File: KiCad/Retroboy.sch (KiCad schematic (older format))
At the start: 1 part, among them J1 1473005-1

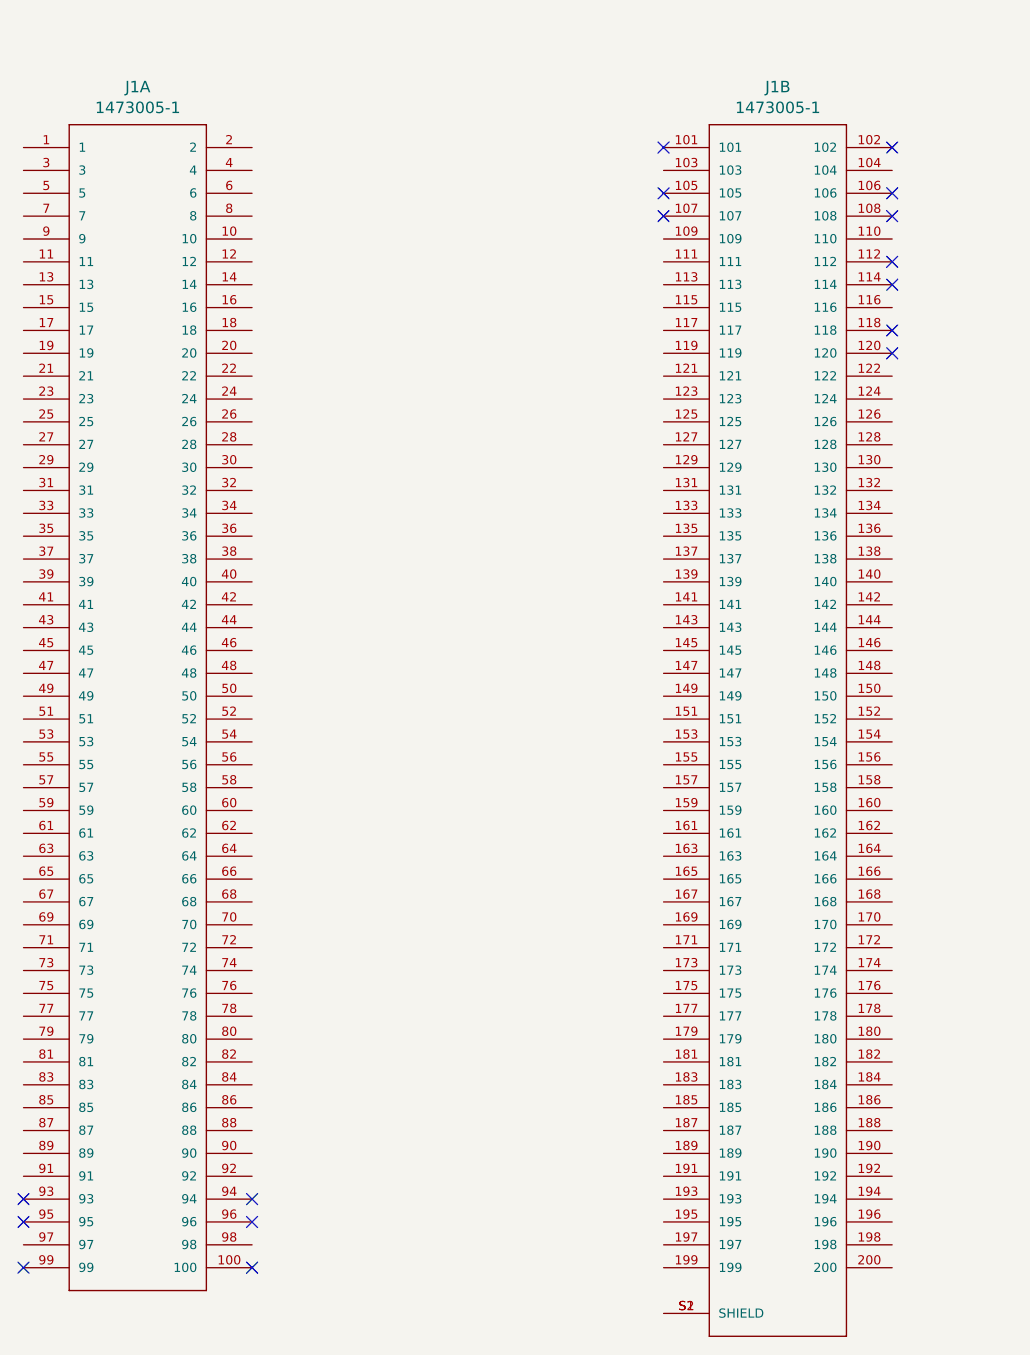
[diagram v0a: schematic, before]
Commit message: Updates.
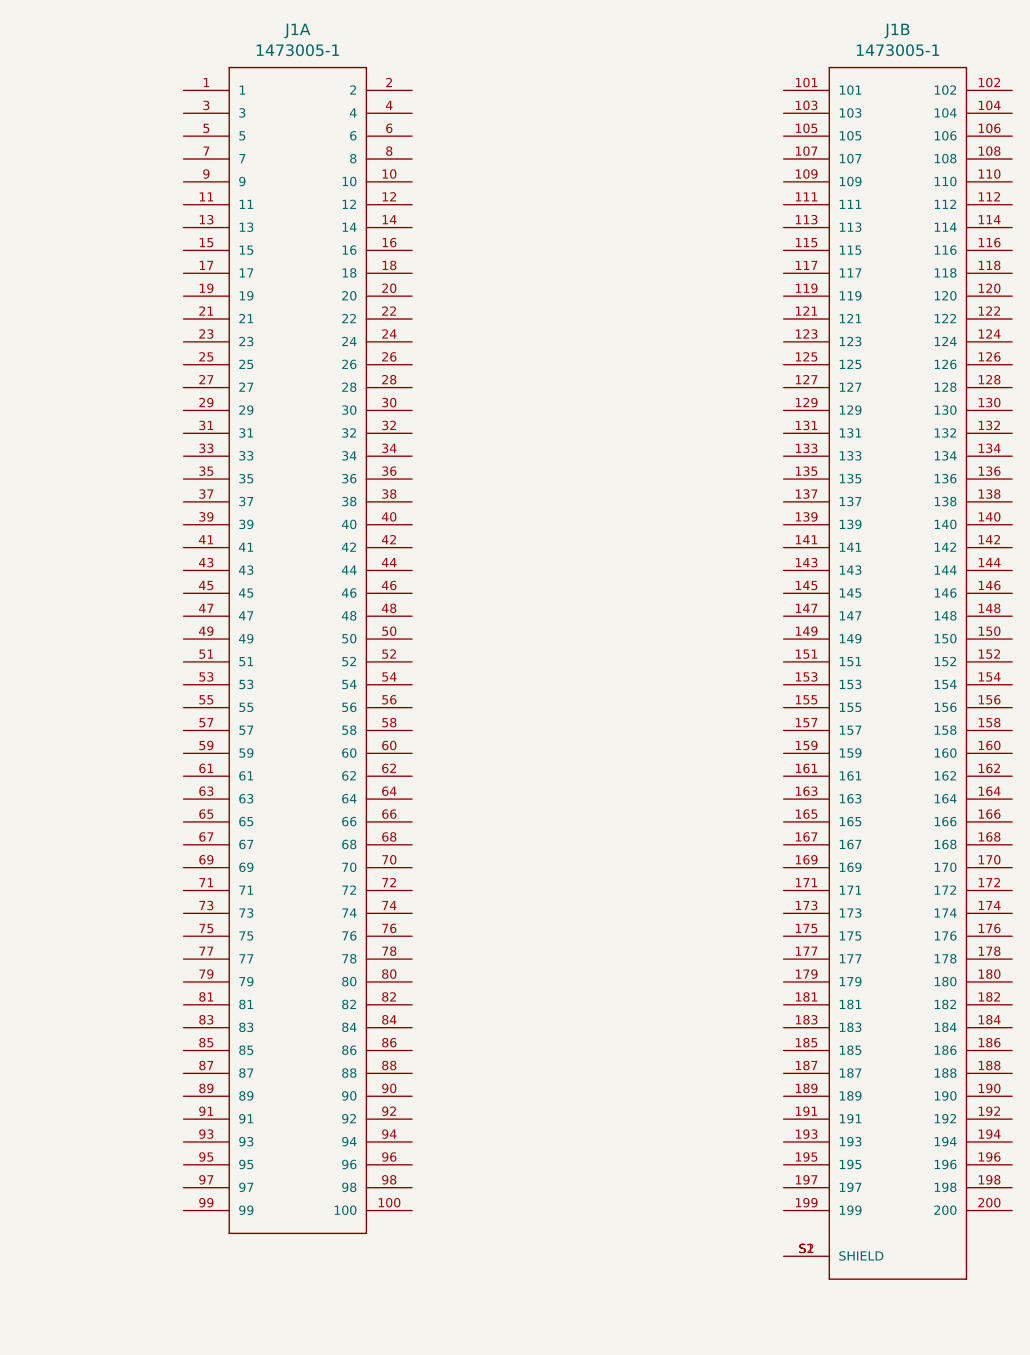
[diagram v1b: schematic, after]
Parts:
- J1: footprint TE_1473005-1:TE_1473005-1 -> TE_1473005-1
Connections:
- no-connect marks 16 -> 0
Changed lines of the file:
@@
 encoding utf-8
 Sheet 1 1
-Title "Raspberry PI Compute 3+ Connector"
+Title "Retroboy - Retro Gaming Console"
 Date ""
 Rev ""
@@
 $Comp
 L 1473005-1:1473005-1 J1
-U 1 1 5F6D85EE
-P 2350 4000
-F 0 "J1" H 2350 6665 50  0000 C CNN
-F 1 "1473005-1" H 2350 6574 50  0000 C CNN
-F 2 "TE_1473005-1:TE_1473005-1" H 2350 4000 50  0001 L BNN
-F 3 "Manufacturer Recommendations" H 2350 4000 50  0001 L BNN
-F 4 "J3" H 2350 4000 50  0001 L BNN "Field4"
-F 5 "TE Connectivity" H 2350 4000 50  0001 L BNN "Field5"
-F 6 "5.9mm" H 2350 4000 50  0001 L BNN "Field6"
-	1    2350 4000
+U 1 1 5F78AB01
+P 3050 3750
+F 0 "J1" H 3050 6415 50  0000 C CNN
+F 1 "1473005-1" H 3050 6324 50  0000 C CNN
+F 2 "TE_1473005-1" H 3050 3750 50  0001 L BNN
+F 3 "Manufacturer Recommendations" H 3050 3750 50  0001 L BNN
+F 4 "J3" H 3050 3750 50  0001 L BNN "Field4"
+F 5 "TE Connectivity" H 3050 3750 50  0001 L BNN "Field5"
+F 6 "5.9mm" H 3050 3750 50  0001 L BNN "Field6"
+	1    3050 3750
 	1    0    0    -1
 $EndComp
 $Comp
 L 1473005-1:1473005-1 J1
-U 2 1 5F6DFEDF
-P 5150 4100
-F 0 "J1" H 5150 6865 50  0000 C CNN
-F 1 "1473005-1" H 5150 6774 50  0000 C CNN
-F 2 "TE_1473005-1:TE_1473005-1" H 5150 4100 50  0001 L BNN
-F 3 "Manufacturer Recommendations" H 5150 4100 50  0001 L BNN
-F 4 "J3" H 5150 4100 50  0001 L BNN "Field4"
-F 5 "TE Connectivity" H 5150 4100 50  0001 L BNN "Field5"
-F 6 "5.9mm" H 5150 4100 50  0001 L BNN "Field6"
-	2    5150 4100
+U 2 1 5F78F8D6
+P 5675 3850
+F 0 "J1" H 5675 6615 50  0000 C CNN
+F 1 "1473005-1" H 5675 6524 50  0000 C CNN
+F 2 "TE_1473005-1" H 5675 3850 50  0001 L BNN
+F 3 "Manufacturer Recommendations" H 5675 3850 50  0001 L BNN
+F 4 "J3" H 5675 3850 50  0001 L BNN "Field4"
+F 5 "TE Connectivity" H 5675 3850 50  0001 L BNN "Field5"
+F 6 "5.9mm" H 5675 3850 50  0001 L BNN "Field6"
+	2    5675 3850
 	1    0    0    -1
 $EndComp
-NoConn ~ 1850 6200
-NoConn ~ 2850 6200
-NoConn ~ 1850 6300
-NoConn ~ 2850 6300
-NoConn ~ 1850 6500
-NoConn ~ 2850 6500
-NoConn ~ 4650 1600
-NoConn ~ 5650 1600
-NoConn ~ 4650 1800
-NoConn ~ 5650 1800
-NoConn ~ 4650 1900
-NoConn ~ 5650 1900
-NoConn ~ 5650 2100
-NoConn ~ 5650 2200
-NoConn ~ 5650 2400
-NoConn ~ 5650 2500
 $EndSCHEMATC
